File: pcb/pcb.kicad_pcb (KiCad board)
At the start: 4 copper layers, 48.3 x 68.5 mm, 54 parts, among them J1 Conn_02x09_Odd_Even, J10 Conn_01x05, J11 Conn_01x02, J12 Conn_01x02, J2 Conn_02x09_Odd_Even, J3 Conn_02x09_Odd_Even, J4 Conn_02x09_Odd_Even, J5 Jack-DC, J6 Conn_01x04, J7 Conn_01x05, J8 Conn_01x01, J9 Conn_01x02, U1 MCP23017, U2 MCP23017, U3 MCP23017, U4 MCP23017, U5 LMZ12002, U6 LMZ12002, U8 TXS0102, X1 PLTWS7, Y1 Mount, Y2 Mount, Y3 Mount, Y4 Mount

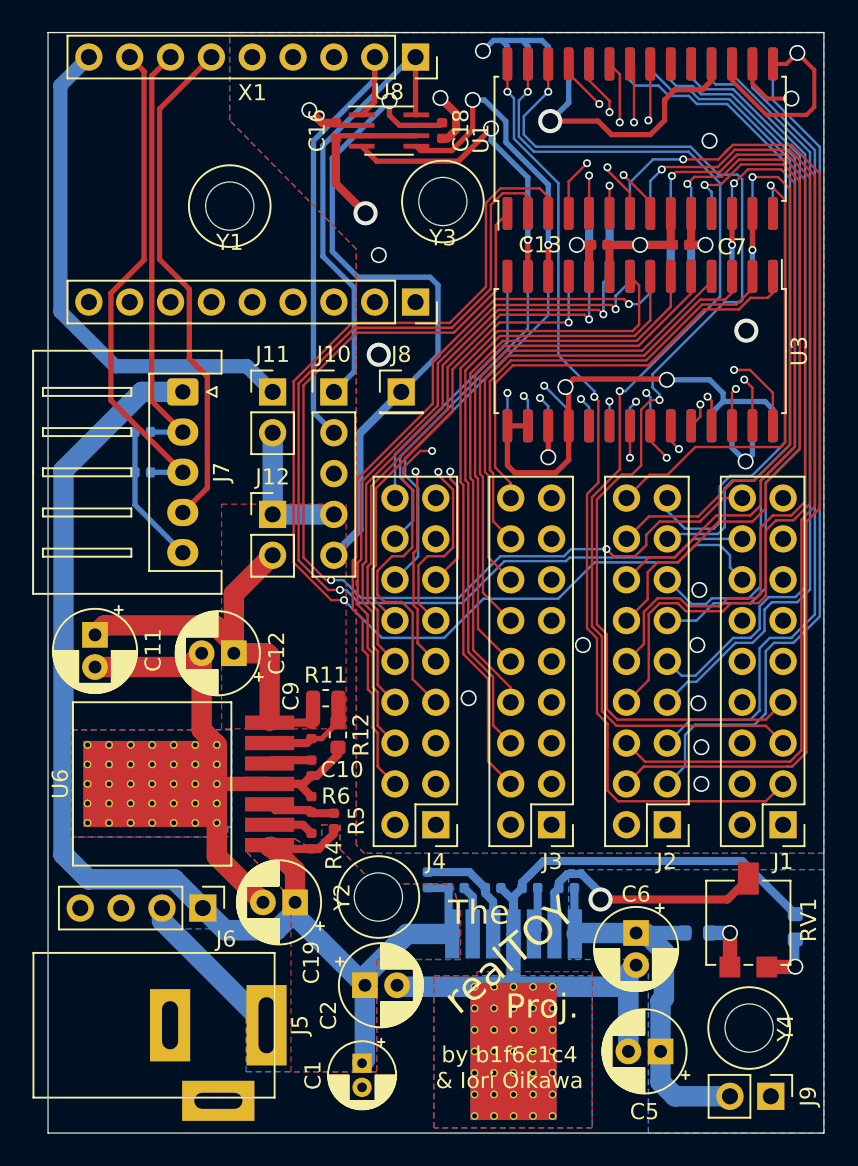
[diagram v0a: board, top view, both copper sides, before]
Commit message: tune
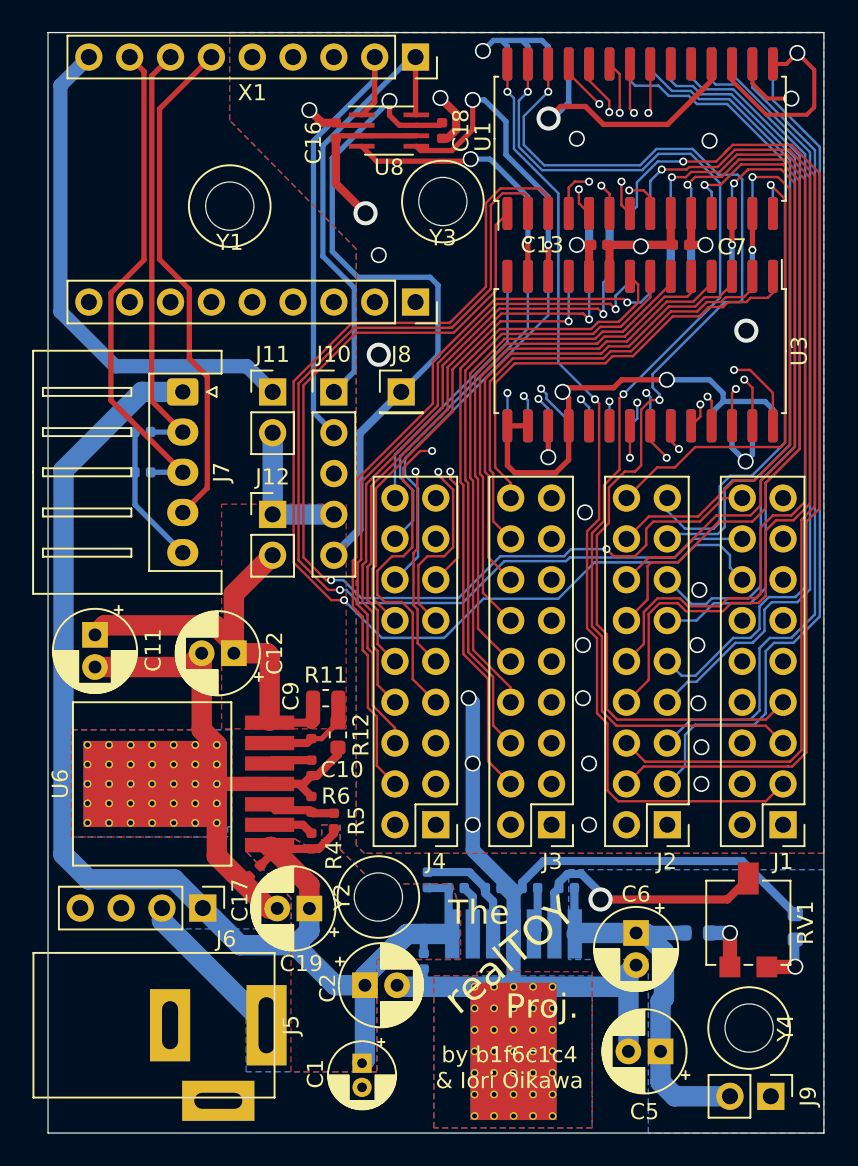
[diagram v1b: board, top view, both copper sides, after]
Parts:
- added C15: 100n, Capacitor_SMD:C_0402_1005Metric, B.Cu at (125.0, 134.0)
- added C17: 100n, Capacitor_SMD:C_0402_1005Metric, F.Cu at (114.5, 128.4)
- moved C19 0.97 mm to (117.9, 130.7)
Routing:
- net GND: track 575.2 -> 582.0 mm, vias 19 -> 26
- net /VIN: track 82.8 -> 87.5 mm
- net /sda: track 38.7 -> 36.0 mm
- net Net-(J1-Pad6): track 49.8 -> 47.7 mm
- net Net-(J1-Pad8): track 48.3 -> 46.9 mm
- net Net-(J1-Pad10): track 48.1 -> 46.7 mm
- net Net-(J1-Pad7): track 70.0 -> 71.2 mm
- net Net-(J1-Pad5): track 67.2 -> 68.2 mm
- net Net-(J1-Pad4): track 50.5 -> 49.6 mm
- net Net-(J3-Pad4): track 42.6 -> 41.7 mm
- net Net-(J3-Pad6): track 39.9 -> 39.0 mm
- net Net-(J3-Pad8): track 37.6 -> 36.7 mm
- net Net-(J1-Pad13): track 44.8 -> 44.0 mm
- net Net-(J1-Pad15): track 40.5 -> 39.7 mm
- net Net-(J1-Pad12): track 44.0 -> 43.4 mm
